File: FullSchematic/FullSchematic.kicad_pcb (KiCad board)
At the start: 4 copper layers, 146 x 132 mm, 100 parts, among them J1 USB_A, J10 LCD_Conn, J2 ATX-24, J3 Red Banana Jack, J4 Black Banana Jack, J5 2x6 Pin Header, J6 2x6 Pin Header, J7 CT3151-2, J8 CT3151-2, J9 2x6 Pin Header, Q1 BSS138-7-F, Q2 BSS138-7-F, Q3 NPN, SW1 Rotary Switch, U1 IR2181STRPBF, U10 SN74LVC2T45DCURE4, U11 SN74LVC2T45DCURE4, U12 SN74LVC2T45DCURE4, U13 SN74LVC2T45DCURE4, U14 SN74LV595ARGYR, U2 IR2181STRPBF, U3 IPB009N03L G, U4 IPB009N03L G, U5 IPB009N03L G, U6 IPB009N03L G, U7 Current Sensor, U8 Op Amp, U9 L79L05ABD13TR

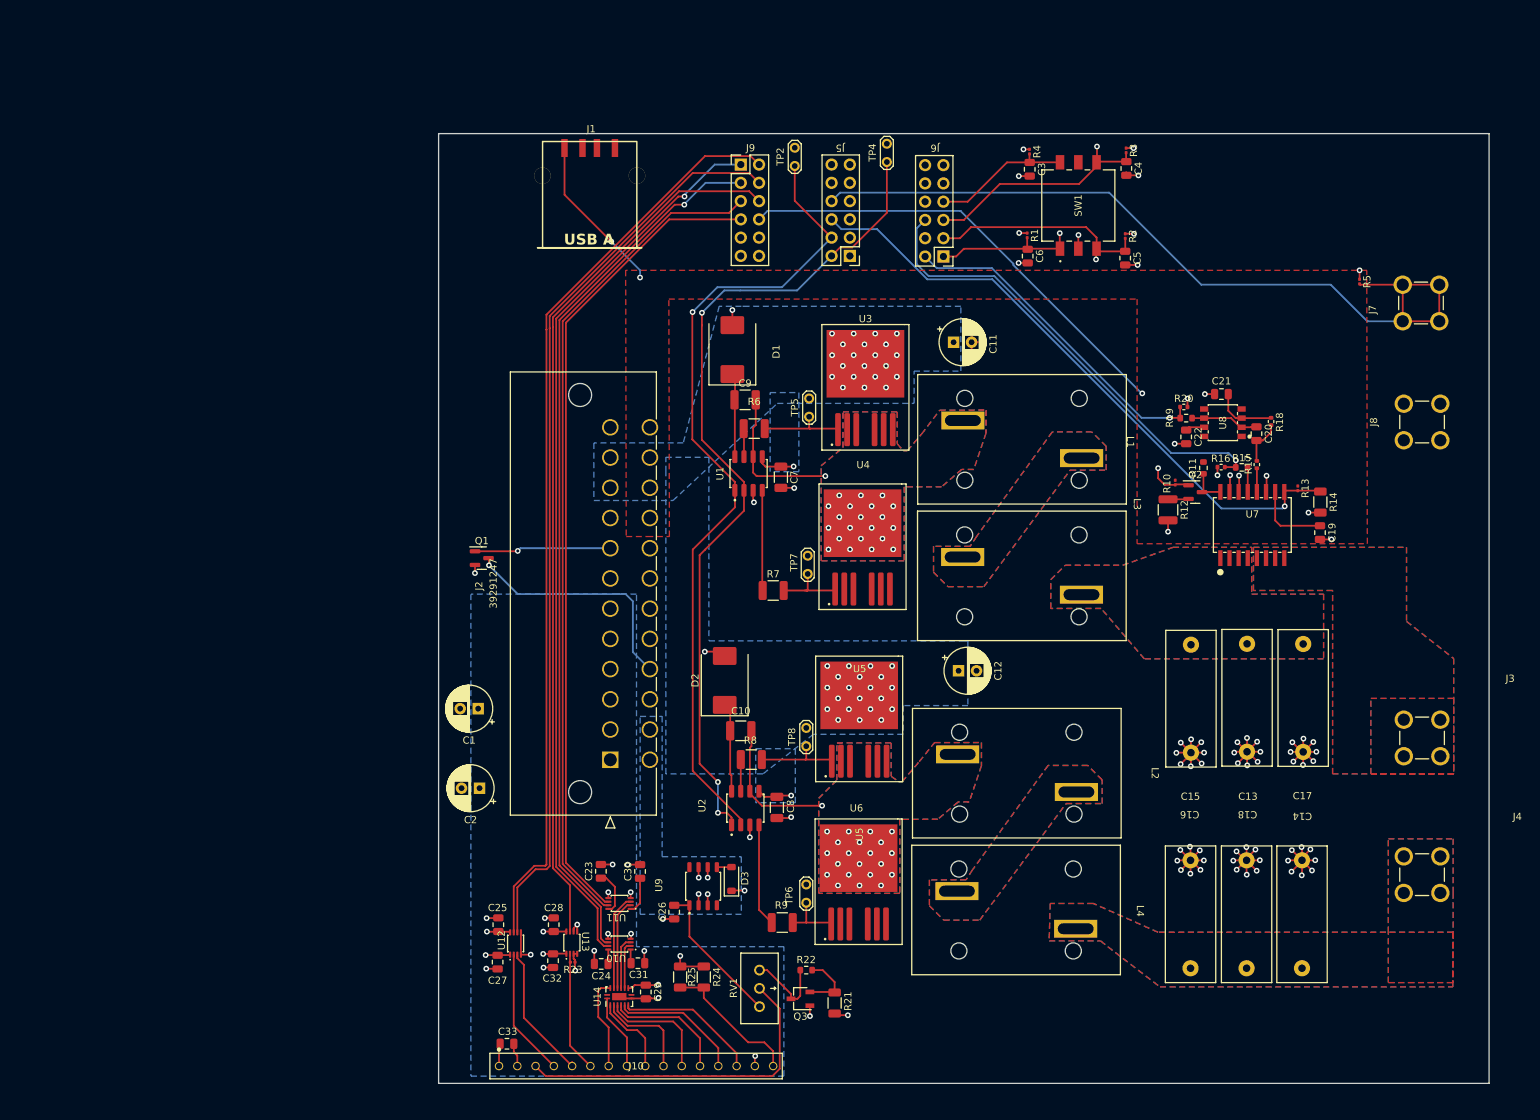
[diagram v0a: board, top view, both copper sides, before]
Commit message: Circuit Board V.2
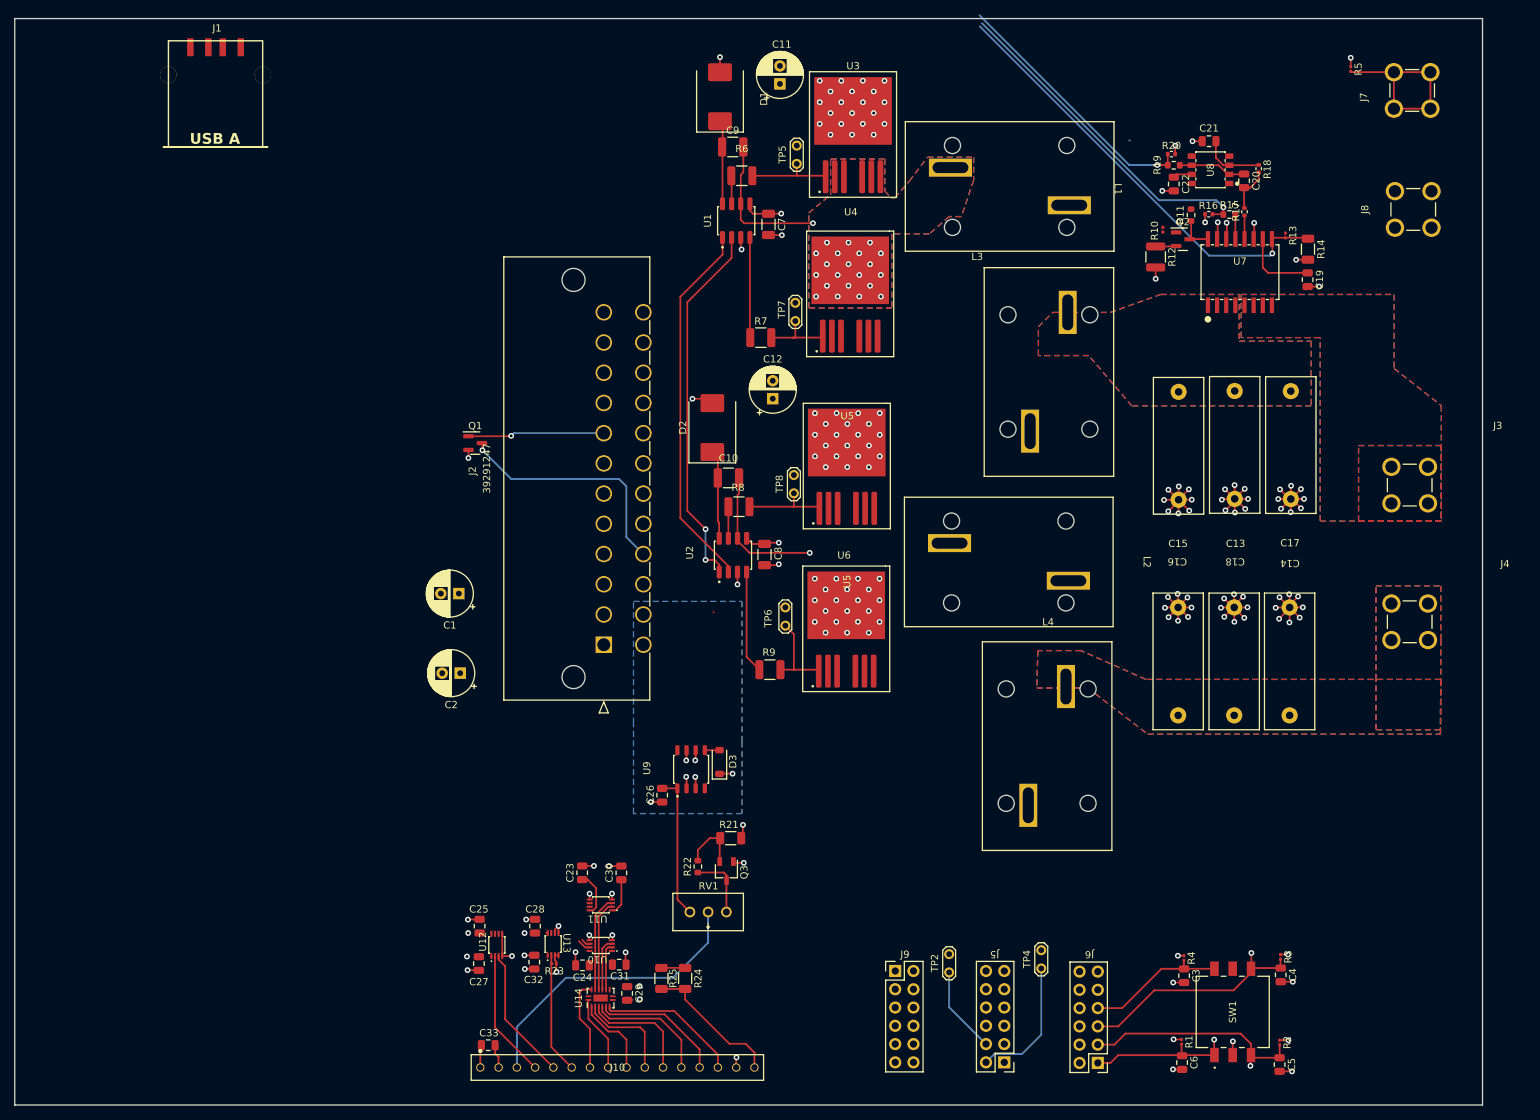
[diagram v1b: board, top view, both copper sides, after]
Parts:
- moved C3 114.1 mm to (180.6, 147.0)
- moved J6 114.1 mm to (167.3, 153.7)
- moved J9 114.1 mm to (141.8, 151.9)
- moved C4 114.1 mm to (194.0, 146.9)
- moved C5 114.1 mm to (193.9, 159.4)
- moved C6 114.1 mm to (180.3, 159.1)
- moved J5 114.1 mm to (154.3, 153.6)
- moved R1 114.1 mm to (180.3, 156.2)
- moved R2 114.1 mm to (193.9, 156.3)
- moved R3 114.1 mm to (194.0, 144.4)
- moved R4 114.1 mm to (180.6, 144.6)
- moved SW1 114.1 mm to (187.4, 152.1)
- moved TP2 114.1 mm to (148.0, 146.6)
- moved TP4 114.1 mm to (160.8, 146.0)
- moved J1 53.9 mm to (46.0, 31.9)
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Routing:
- net Net-(U12-B1): track 127.8 -> 0.00 mm
- net Net-(U12-B2): track 126.3 -> 0.00 mm
- net SRCLK: track 125.2 -> 1.84 mm, vias 1 -> 0
- net Net-(U13-B1): track 122.8 -> 0.00 mm
- net RCLK: track 122.8 -> 1.26 mm, vias 1 -> 0
- net *OE: track 115.8 -> 0.00 mm
- net SER: track 113.5 -> 0.00 mm
- net RELAY_TRIP_N: track 113.6 -> 26.4 mm
- net OC_RESET_N: track 81.8 -> 0.48 mm, vias 2 -> 0
- net NON_INV: track 114.9 -> 64.0 mm, vias 1 -> 0
- net INV: track 117.6 -> 70.5 mm, vias 3 -> 2
- net +5V: track 60.6 -> 27.4 mm, vias 6 -> 3
- net FAULT_N: track 86.9 -> 61.1 mm
- net C_REF: track 64.8 -> 46.7 mm
- net COM: track 172.1 -> 162.0 mm, vias 91 -> 88
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- removed copper zone on B.Cu, net +12V
- removed copper zone on In2.Cu, net +3.3V
- removed copper zone on B.Cu, net +5V
- removed copper zone on F.Cu, net +5V
- removed copper zone on In1.Cu, net COM
- removed copper zone on B.Cu, net Net-(L1-Pad2)
- removed copper zone on F.Cu, net Net-(L1-Pad2)
- removed copper zone on In1.Cu, net Net-(L1-Pad2)
- removed copper zone on In2.Cu, net Net-(L1-Pad2)
- removed copper zone on B.Cu, net Net-(L2-Pad2)
- removed copper zone on F.Cu, net Net-(L2-Pad2)
- removed copper zone on In1.Cu, net Net-(L2-Pad2)
- removed copper zone on In2.Cu, net Net-(L2-Pad2)
- removed copper zone on B.Cu, net Net-(U2-VS)
- removed copper zone on F.Cu, net Net-(U2-VS)
- removed copper zone on In1.Cu, net Net-(U2-VS)
- removed copper zone on In2.Cu, net Net-(U2-VS)
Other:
- board size 146 x 132 mm -> 204 x 151 mm
